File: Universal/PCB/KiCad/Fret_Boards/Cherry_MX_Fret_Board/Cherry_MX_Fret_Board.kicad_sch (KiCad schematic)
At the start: 16 parts, among them SW1 MX_SW_HS, SW2 MX_SW_HS, SW3 MX_SW_HS, SW4 MX_SW_HS, SW5 MX_SW_HS

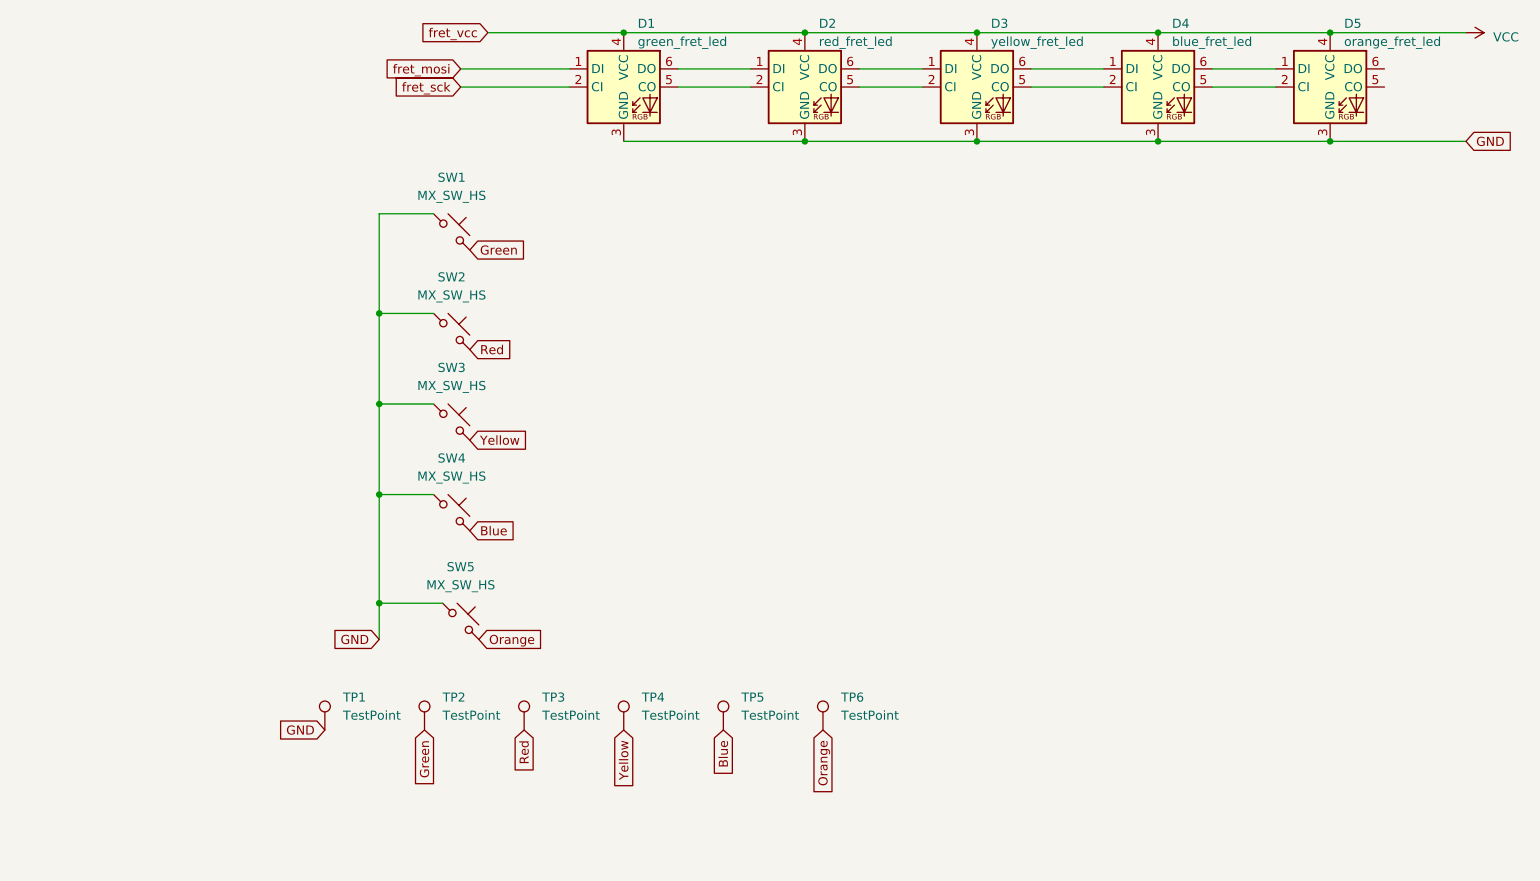
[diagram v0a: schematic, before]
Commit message: updated the MX fret board
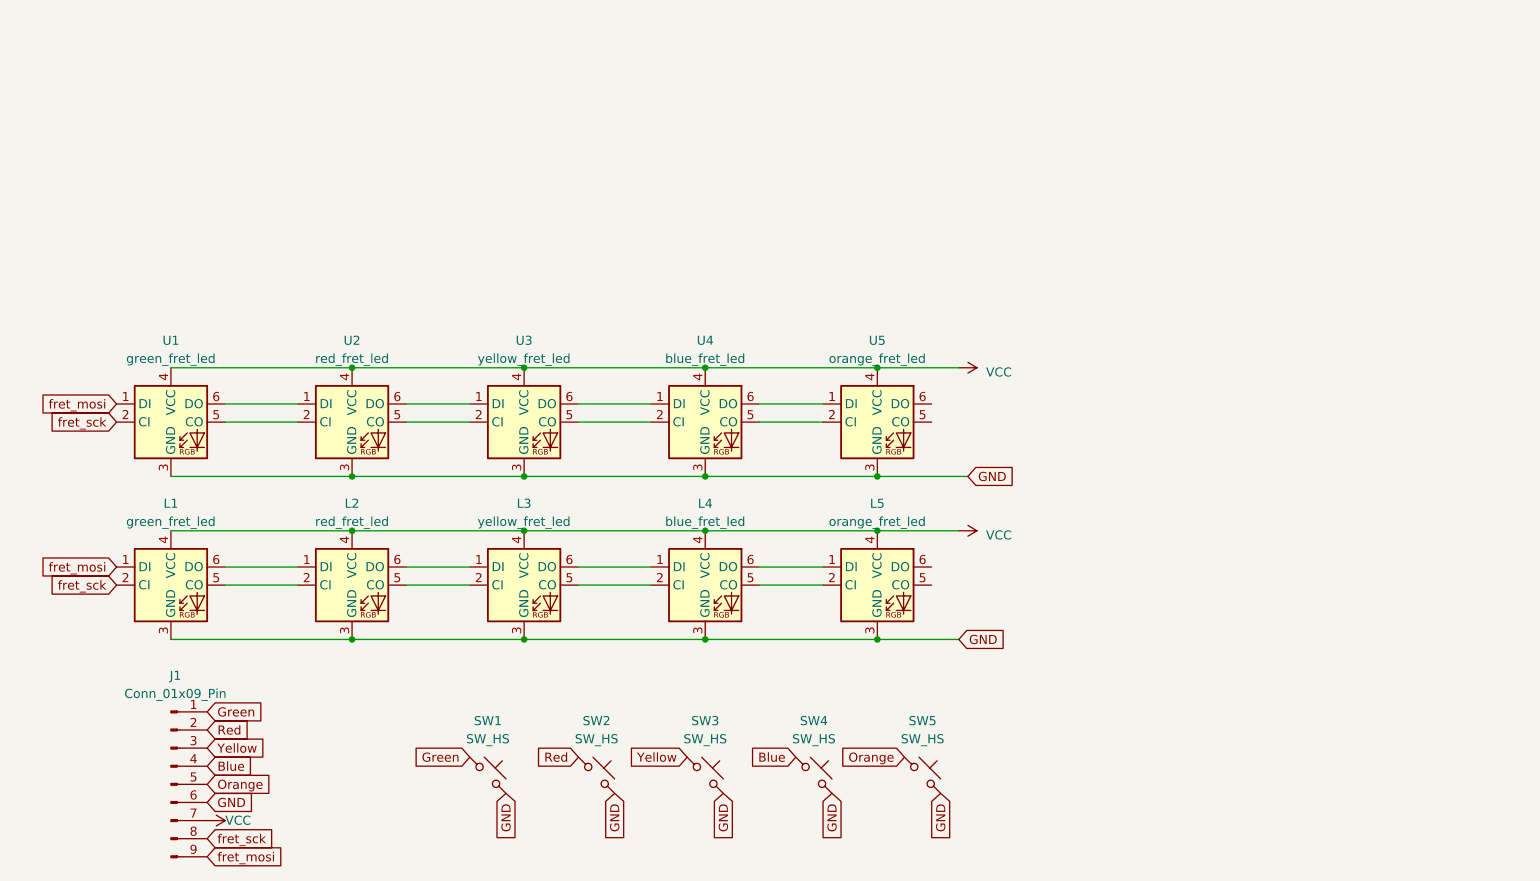
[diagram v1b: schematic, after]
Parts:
- removed TP1, TP2, TP3, TP4, TP5, TP6: TestPoint, symbol Connector:TestPoint
- added J1: Conn_01x09_Pin, Connector_PinHeader_2.54mm:PinHeader_1x09_P2.54mm_Vertical, symbol Connector:Conn_01x09_Pin
- added U1: green_fret_led, LED_SMD:LED_RGB_5050-6, symbol LED:APA102
- added U2: red_fret_led, LED_SMD:LED_RGB_5050-6, symbol LED:APA102
- added U3: yellow_fret_led, LED_SMD:LED_RGB_5050-6, symbol LED:APA102
- added U4: blue_fret_led, LED_SMD:LED_RGB_5050-6, symbol LED:APA102
- added U5: orange_fret_led, LED_SMD:LED_RGB_5050-6, symbol LED:APA102
- SW1, SW2, SW3, SW4, SW5: value MX_SW_HS -> SW_HS; footprint marbastlib-mx:SW_MX_HS_1u -> Minibar:Kailh_Hotswap_MX
- renumbered D1 to L1, D2 to L2, D3 to L3, D4 to L4, D5 to L5
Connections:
- net Blue: now also SW4.1, J1.4 (Pin_4); no longer SW4.2
- net GND: now also SW1.2, SW2.2, SW3.2, SW4.2, SW5.2, J1.6 (Pin_6), U1.3 (GND), U2.3 (GND), U3.3 (GND), U4.3 (GND), U5.3 (GND); no longer SW1.1, SW2.1, SW3.1, SW4.1, SW5.1
- net Green: now also SW1.1, J1.1 (Pin_1); no longer SW1.2
- net Orange: now also SW5.1, J1.5 (Pin_5); no longer SW5.2
- net Red: now also SW2.1, J1.2 (Pin_2); no longer SW2.2
- net VCC: now also J1.7 (Pin_7), U1.4 (VCC), U2.4 (VCC), U3.4 (VCC), U4.4 (VCC), U5.4 (VCC)
- net Yellow: now also SW3.1, J1.3 (Pin_3); no longer SW3.2
- net fret_mosi: now also J1.9 (Pin_9), U1.1 (DI)
- net fret_sck: now also J1.8 (Pin_8), U1.2 (CI)
- new net: U1.6 (DO), U2.1 (DI)
- new net: U1.5 (CO), U2.2 (CI)
- new net: U2.5 (CO), U3.2 (CI)
- new net: U2.6 (DO), U3.1 (DI)
- new net: U3.5 (CO), U4.2 (CI)
- new net: U3.6 (DO), U4.1 (DI)
- new net: U4.5 (CO), U5.2 (CI)
- new net: U4.6 (DO), U5.1 (DI)
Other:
- moved on the sheet: L1, L2, L3, L4, L5, SW1, SW2, SW3, SW4, SW5
